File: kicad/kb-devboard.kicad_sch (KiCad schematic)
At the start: 121 parts, among them J1 Conn_01x14_Pin, SW1 PG1350, SW10 PG1350, SW11 PG1350, SW12 PG1350, SW13 PG1350, SW14 PG1350, SW15 PG1350, SW16 PG1350, SW17 PG1350, SW18 PG1350, SW19 PG1350, SW2 PG1350, SW20 PG1350, SW21 PG1350, SW22 PG1350, SW23 PG1350, SW24 PG1350, SW25 PG1350, SW26 PG1350, SW27 PG1350, SW28 PG1350, SW29 PG1350, SW3 PG1350, SW30 PG1350, SW4 PG1350, SW5 PG1350, SW6 PG1350, SW7 PG1350, SW8 PG1350, SW9 PG1350

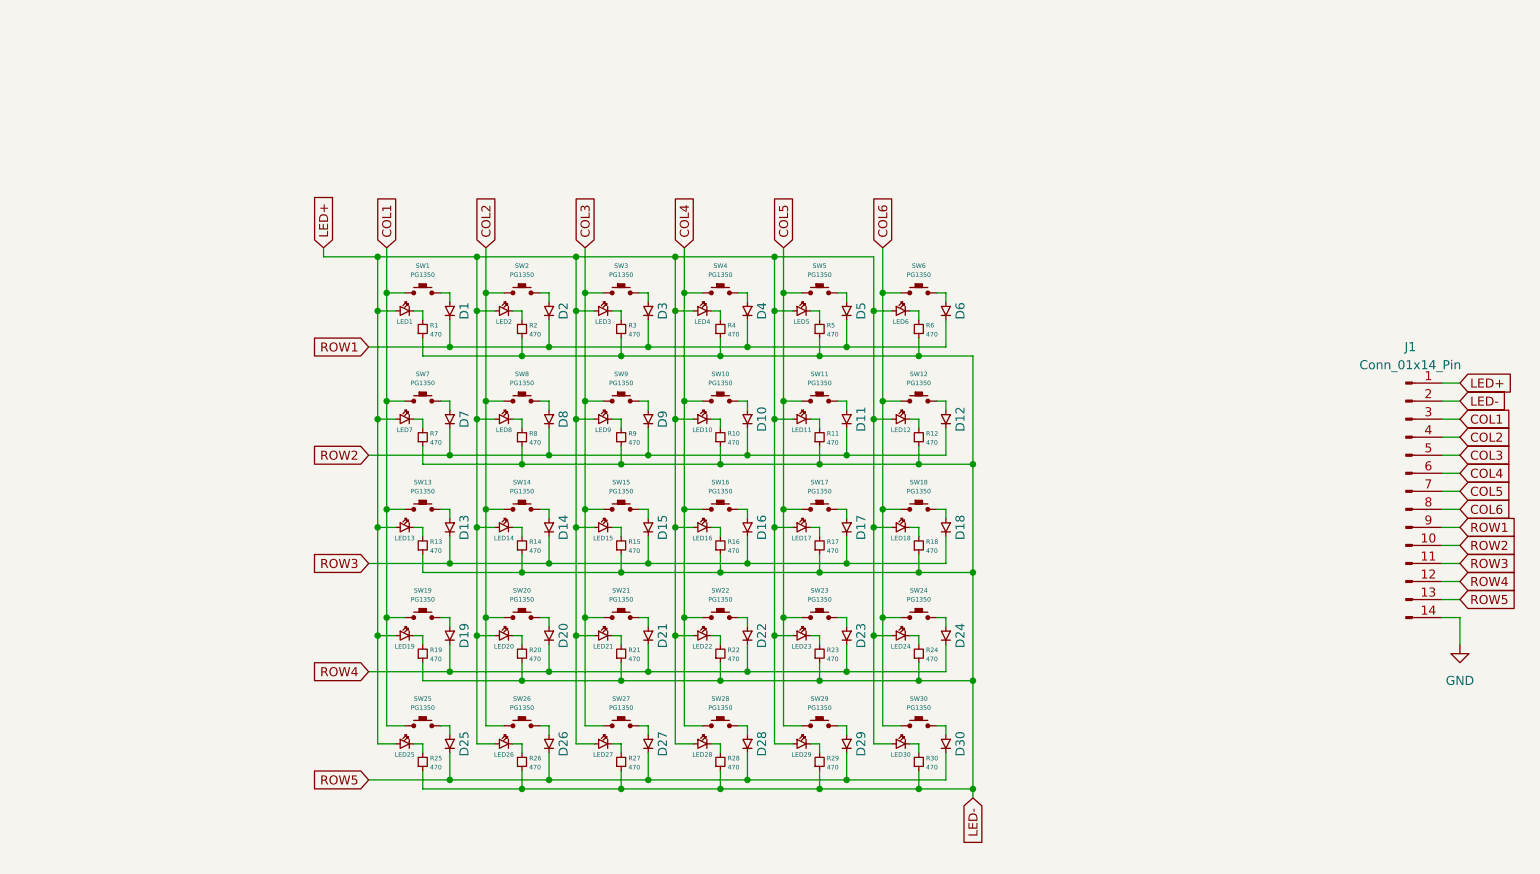
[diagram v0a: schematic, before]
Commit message: Update to rev b
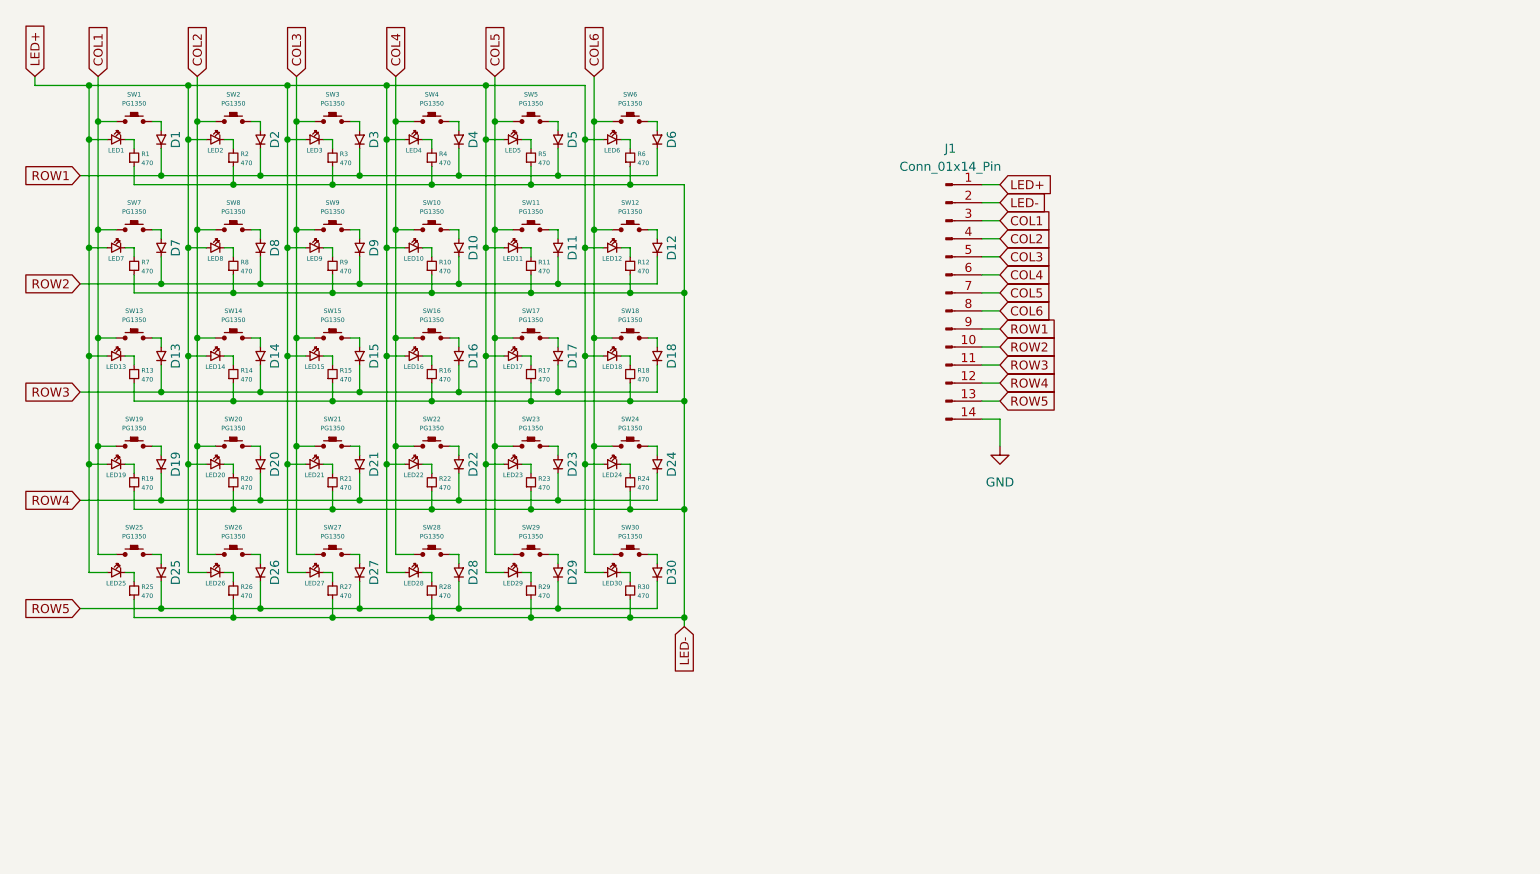
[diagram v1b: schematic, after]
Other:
- moved on the sheet: D1, D10, D11, D12, D13, D14, D15, D16, D17, D18, D19, D2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
